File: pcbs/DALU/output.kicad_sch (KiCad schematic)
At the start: 5 parts, among them U601 74HCT541, U602 74HCT541, U603 74LS540, U604 74HCT541, U605 74HCT541

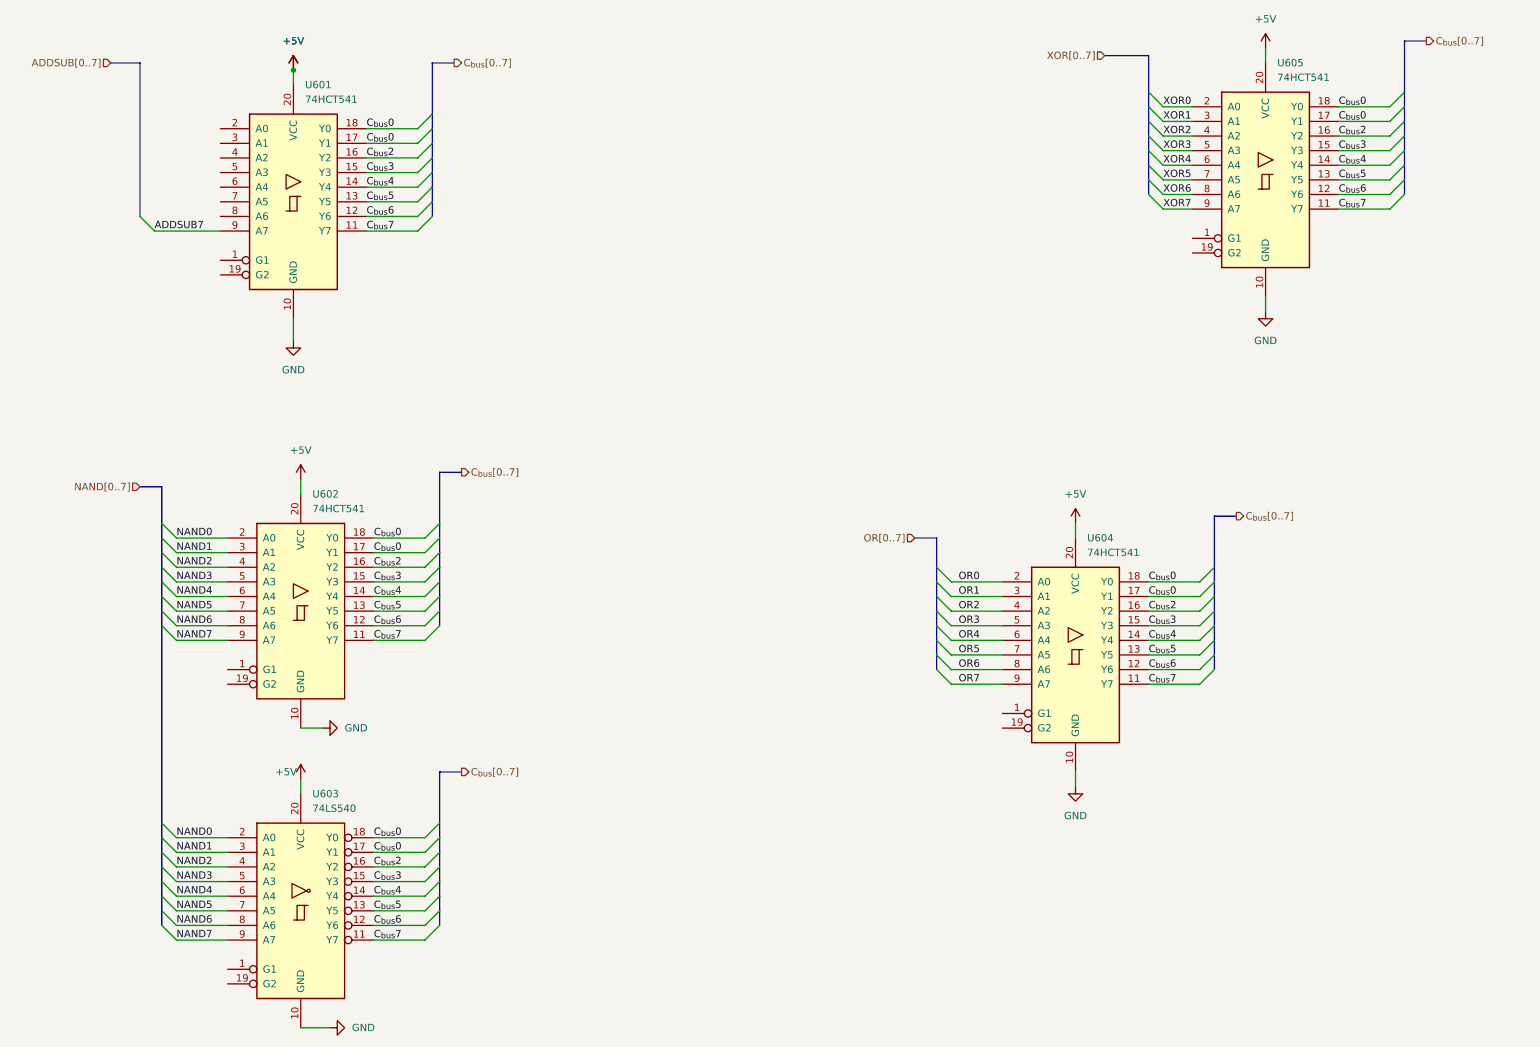
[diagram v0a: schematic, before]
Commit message: Rethinking some design
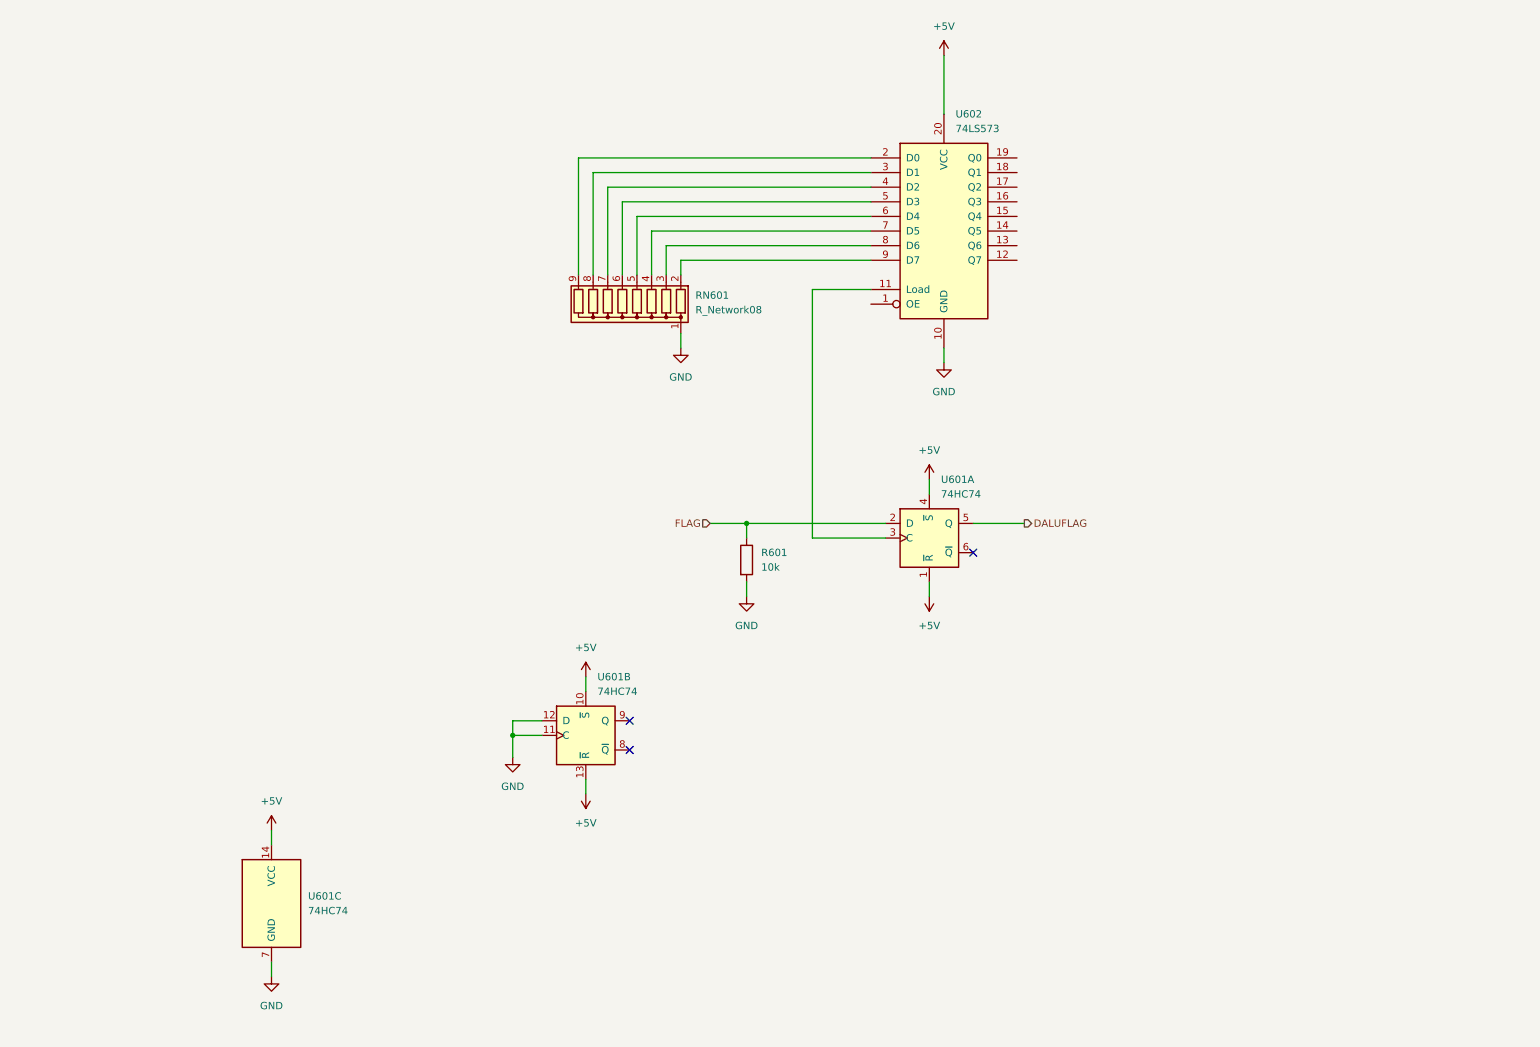
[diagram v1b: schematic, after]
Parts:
- removed U601, U602, U604, U605: 74HCT541, Package_DIP:DIP-20_W7.62mm_Socket, symbol 74xx:74HCT541
- removed U603: 74LS540, Package_DIP:DIP-20_W7.62mm_Socket, symbol 74xx:74LS540
- added R601: 10k, Resistor_THT:R_Axial_DIN0207_L6.3mm_D2.5mm_P7.62mm_Horizontal, symbol Device:R
- added RN601: R_Network08, Resistor_THT:R_Array_SIP9, symbol Device:R_Network08
- added U601: 74HC74, symbol 74xx:74HC74
- added U602: 74LS573, Package_DIP:DIP-20_W7.62mm_Socket, symbol 74xx:74LS573
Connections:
- net +5V: now also U601.1 (~{R}), U601.10 (~{S}), U601.13 (~{R}), U601.14 (VCC), U601.4 (~{S}), U602.20 (VCC)
- net GND: now also R601.2, RN601.1 (common), U601.11 (C), U601.12 (D), U601.7 (GND), U602.10 (GND)
- new net: U601.3 (C), U602.11 (Load)
- new net: RN601.9 (R8), U602.2 (D0)
- new net: RN601.8 (R7), U602.3 (D1)
- new net: RN601.7 (R6), U602.4 (D2)
- new net: RN601.6 (R5), U602.5 (D3)
- new net: RN601.5 (R4), U602.6 (D4)
- new net: RN601.4 (R3), U602.7 (D5)
- new net: RN601.3 (R2), U602.8 (D6)
- new net: RN601.2 (R1), U602.9 (D7)
- new net DALUFLAG: U601.5 (Q)
- new net FLAG: R601.1, U601.2 (D)
- no-connect marks 0 -> 3
